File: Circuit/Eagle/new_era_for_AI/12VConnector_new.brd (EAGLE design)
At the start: 29.5 x 18.5 mm, 10 parts

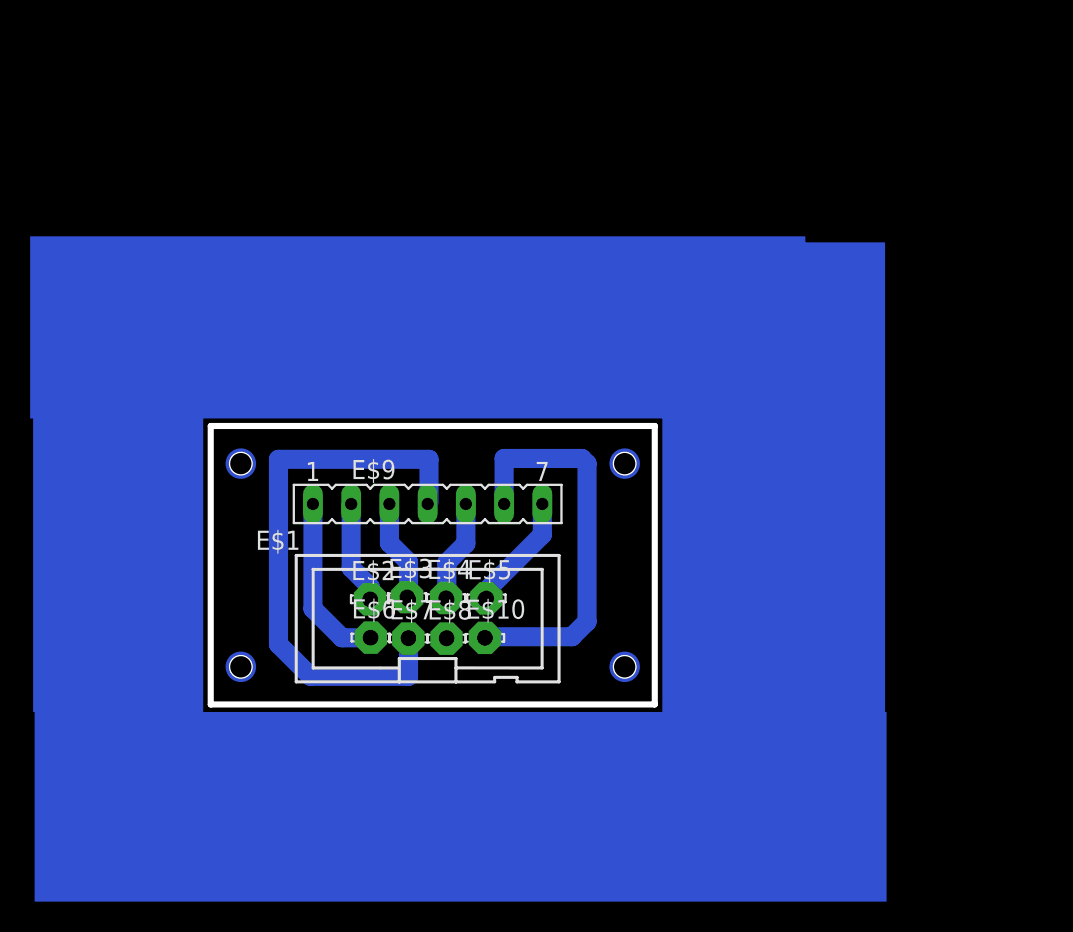
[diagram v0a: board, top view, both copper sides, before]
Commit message: .
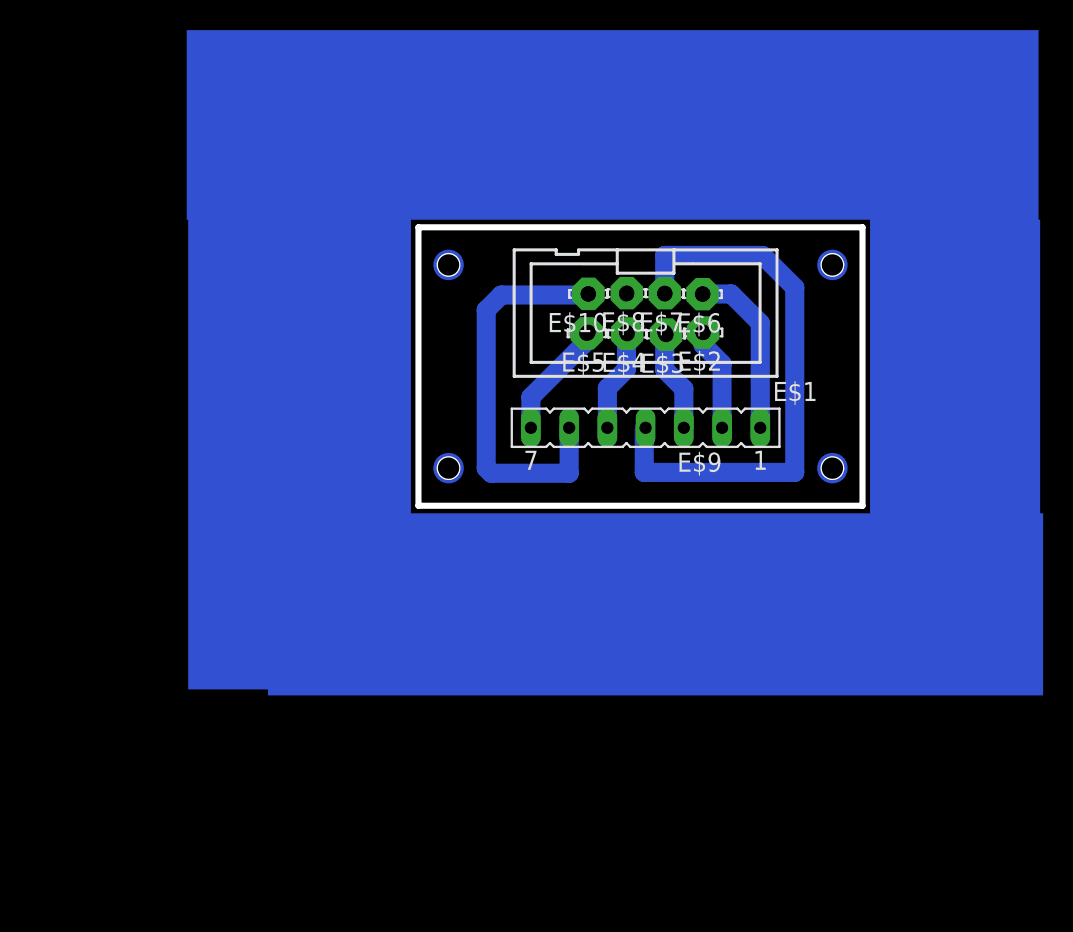
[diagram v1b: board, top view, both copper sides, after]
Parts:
- moved E$6 31.7 mm to (34.2, 28.3), turned to 180 degrees
- moved E$7 28.6 mm to (31.7, 28.3), turned to 180 degrees
- moved E$2 28.3 mm to (34.2, 25.7), turned to 180 degrees
- moved E$1 26.5 mm to (31.7, 27.0), turned to 180 degrees
- moved E$8 25.9 mm to (29.1, 28.3), turned to 180 degrees
- moved E$3 24.5 mm to (31.7, 25.6), turned to 180 degrees
- moved E$10 23.9 mm to (26.6, 28.3), turned to 180 degrees
- moved E$4 21.3 mm to (29.2, 25.6), turned to 180 degrees
- moved E$5 18.8 mm to (26.5, 25.7), turned to 180 degrees
- moved E$9 15.3 mm to (30.4, 19.4), turned to 180 degrees
